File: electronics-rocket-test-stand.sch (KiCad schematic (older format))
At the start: 14 parts

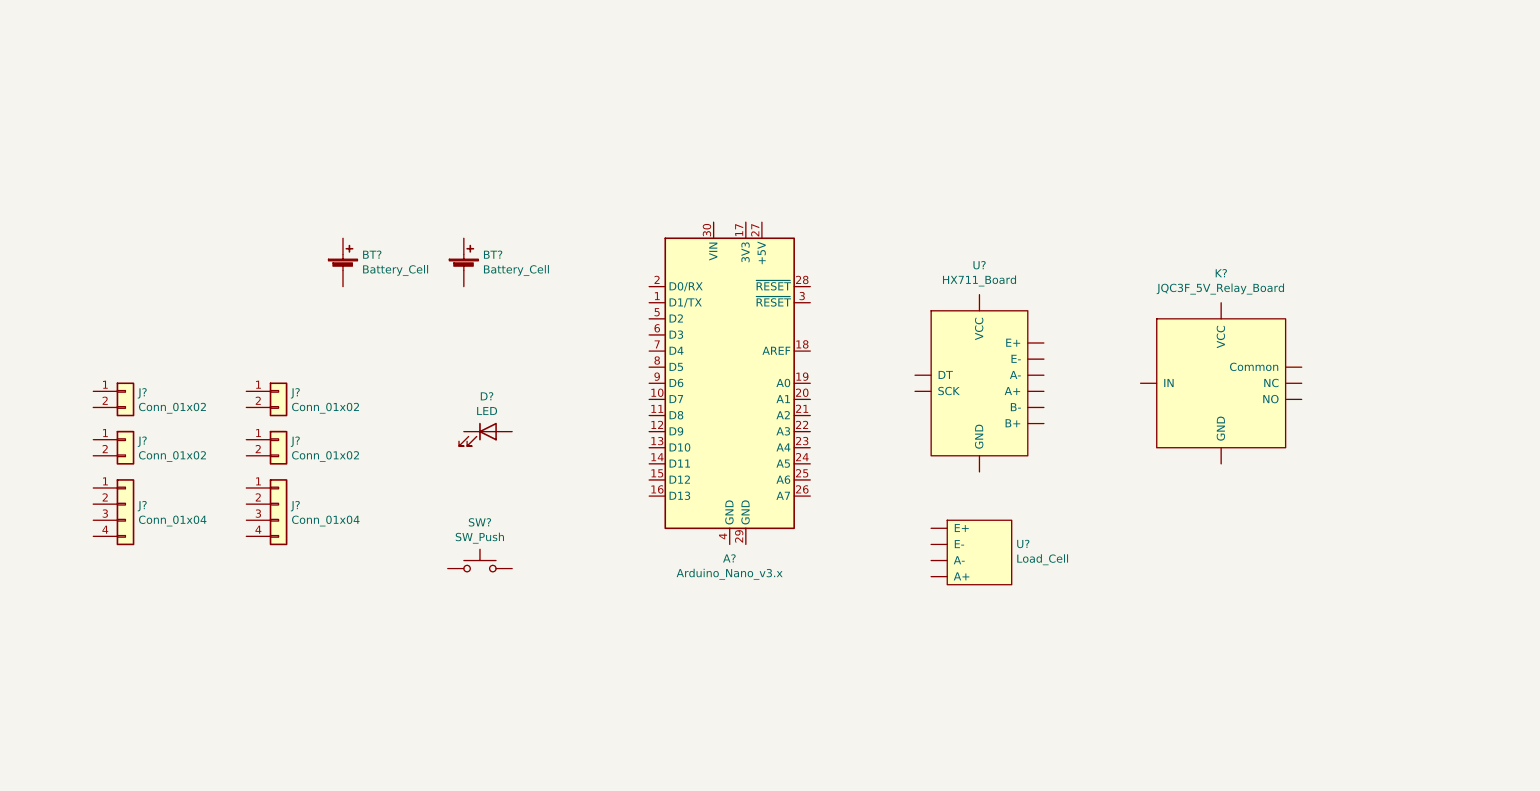
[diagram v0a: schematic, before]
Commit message: Finalize schematic and annotate.
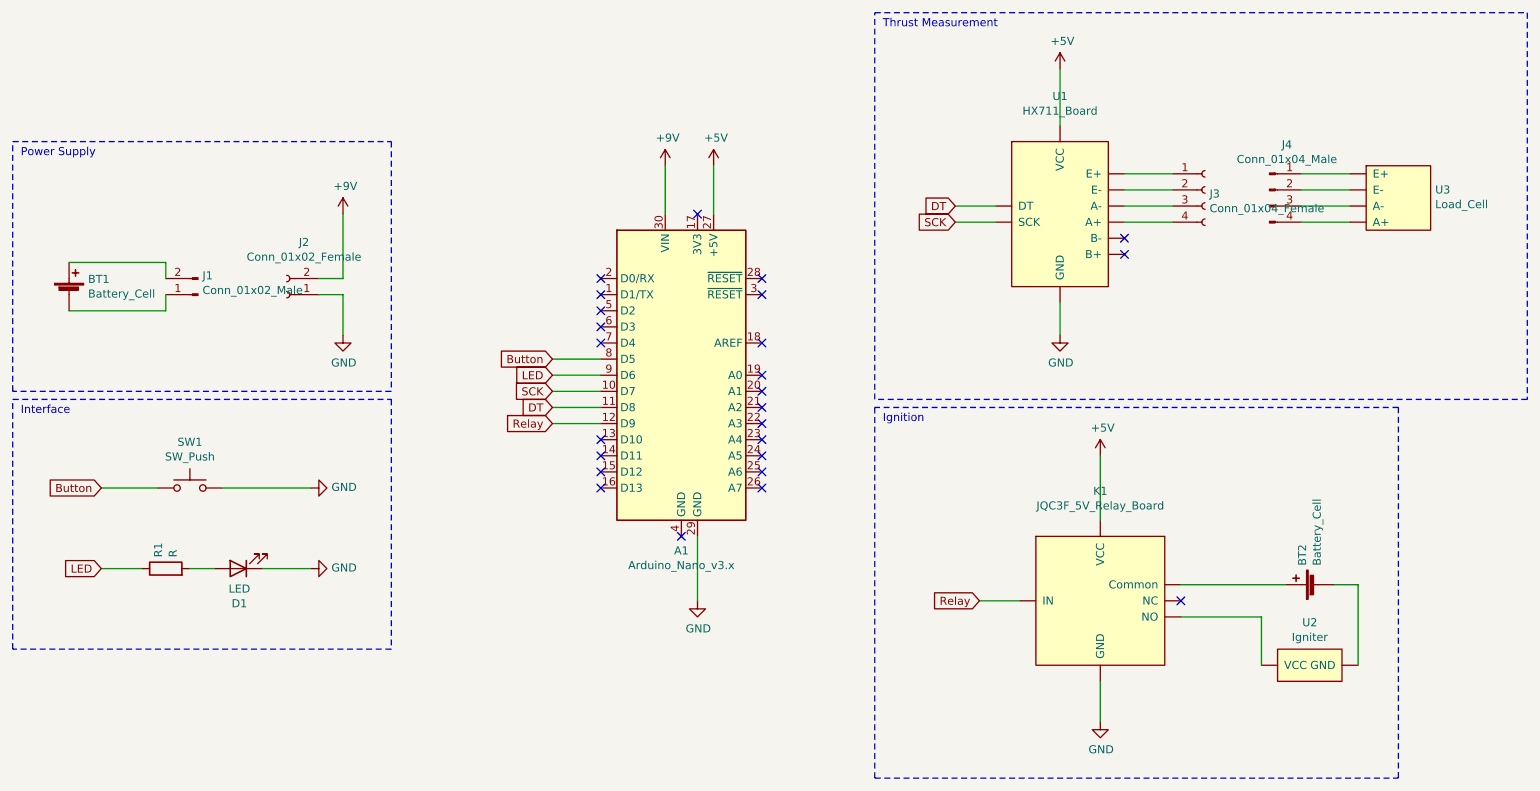
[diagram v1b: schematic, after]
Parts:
- removed J? (x4): Conn_01x02, symbol Connector_Generic:Conn_01x02
- removed J? (x2): Conn_01x04, symbol Connector_Generic:Conn_01x04
- added J1: Conn_01x02_Male, symbol Connector:Conn_01x02_Male
- added J2: Conn_01x02_Female, symbol Connector:Conn_01x02_Female
- added J3: Conn_01x04_Female, symbol Connector:Conn_01x04_Female
- added J4: Conn_01x04_Male, symbol Connector:Conn_01x04_Male
- added R1: R, symbol Device:R
- added U2: Igniter, symbol electronics-rocket-test-stand:Igniter
- gave numbers to parts that had none: 8
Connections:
- net SCK: now reaches A1.10 (D7)
- net SCK: now also U1.~ (VCC)
- net DT: now reaches A1.11 (D8)
- net DT: now also U1.~ (VCC)
- net Relay: now reaches A1.12 (D9)
- net Relay: now also K1.~ (VCC)
- net +5V: now reaches A1.27 (+5V)
- net +5V: now also K1.~ (VCC), U1.~ (VCC)
- net GND: now reaches A1.29 (GND)
- net GND: now also D1.1 (K), K1.~ (VCC), SW1.2, U1.~ (VCC), J2.1 (Pin_1)
- net +9V: now reaches A1.30 (VIN)
- net +9V: now also J2.2 (Pin_2)
- net Button: now reaches A1.8 (D5)
- net Button: now also SW1.1
- net LED: now reaches A1.9 (D6)
- net LED: now also R1.1
- net at BT2.1 (+): now also K1.~ (VCC)
- net at BT2.2 (-): now also U2.~ (VCC)
- net at D1.2 (A): now also R1.2
- net at BT1.1 (+): now also J1.2 (Pin_2)
- net at BT1.2 (-): now also J1.1 (Pin_1)
- net at U3.~ (E-): now also J4.4 (Pin_4)
- new net: J3.1 (Pin_1), U1.~ (VCC)
- new net: J3.2 (Pin_2), U1.~ (VCC)
- new net: J3.3 (Pin_3), U1.~ (VCC)
- new net: J3.4 (Pin_4), U1.~ (VCC)
- new net: K1.~ (VCC), U2.~ (VCC)
- new net: J4.1 (Pin_1), U3.~ (E-)
- new net: J4.2 (Pin_2), U3.~ (E-)
- new net: J4.3 (Pin_3), U3.~ (E-)
- no-connect marks 0 -> 25
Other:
- note added: "Ignition"
- note added: "Interface"
- note added: "Power Supply"
- note added: "Thrust Measurement"
- moved on the sheet: A1, BT1, BT2, D1, K1, SW1, U1, U3
